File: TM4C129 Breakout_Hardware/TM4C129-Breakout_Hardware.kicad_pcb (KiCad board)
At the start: 2 copper layers, 63.5 x 47 mm, 51 parts, among them J1 RJ45, J2 Conn_02x08, J3 Conn_02x08, J4 Conn_02x08, J5 Conn_02x02, J6 Conn_02x02, U1 HX1198FNL, U2 TM4C129ENCPDT, Y1 NX3225GA, Y2 Crystal 32K SMD

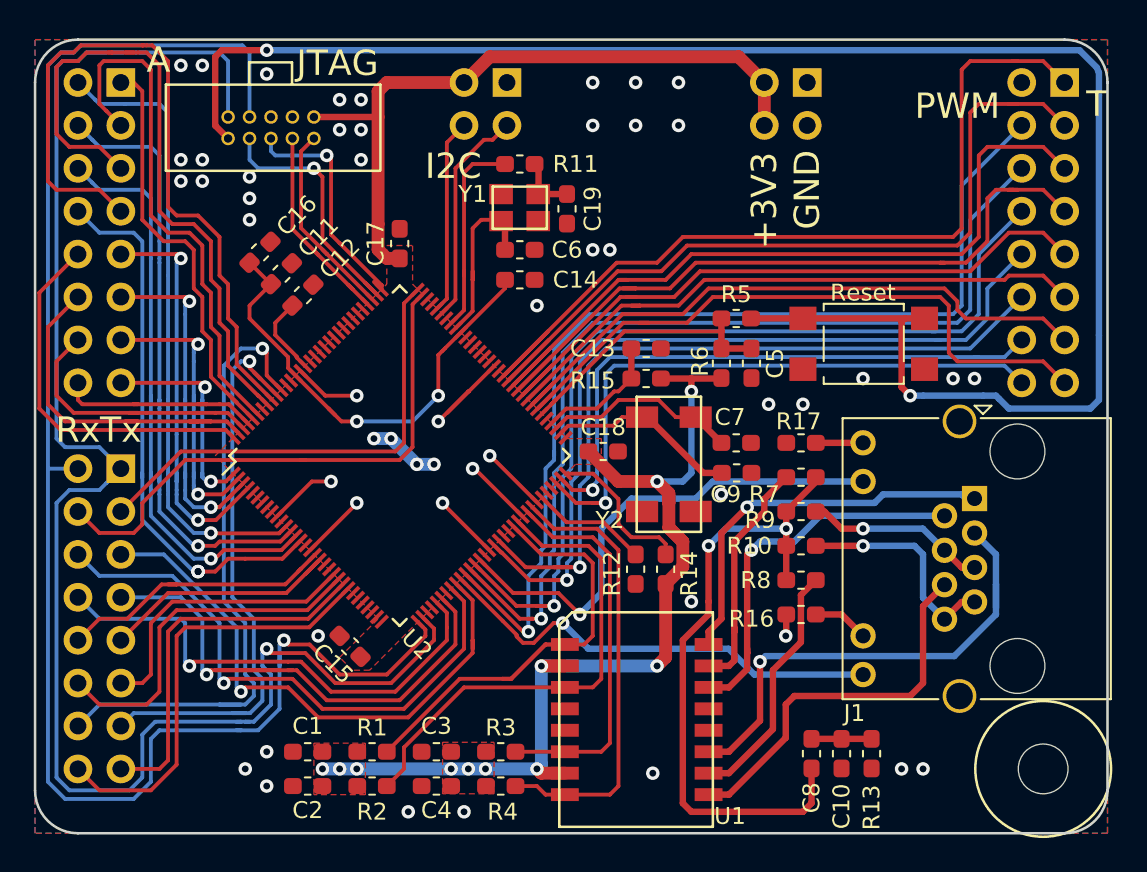
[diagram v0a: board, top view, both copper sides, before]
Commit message: Revert "Revert "Merge branch 'master' of https://github.com/MissouriMRDT/TM4C129-Breakout_Hardware""
This reverts commit 4686fe645caf3e9fbf8c00f0c0ea95986b0ea6b8.
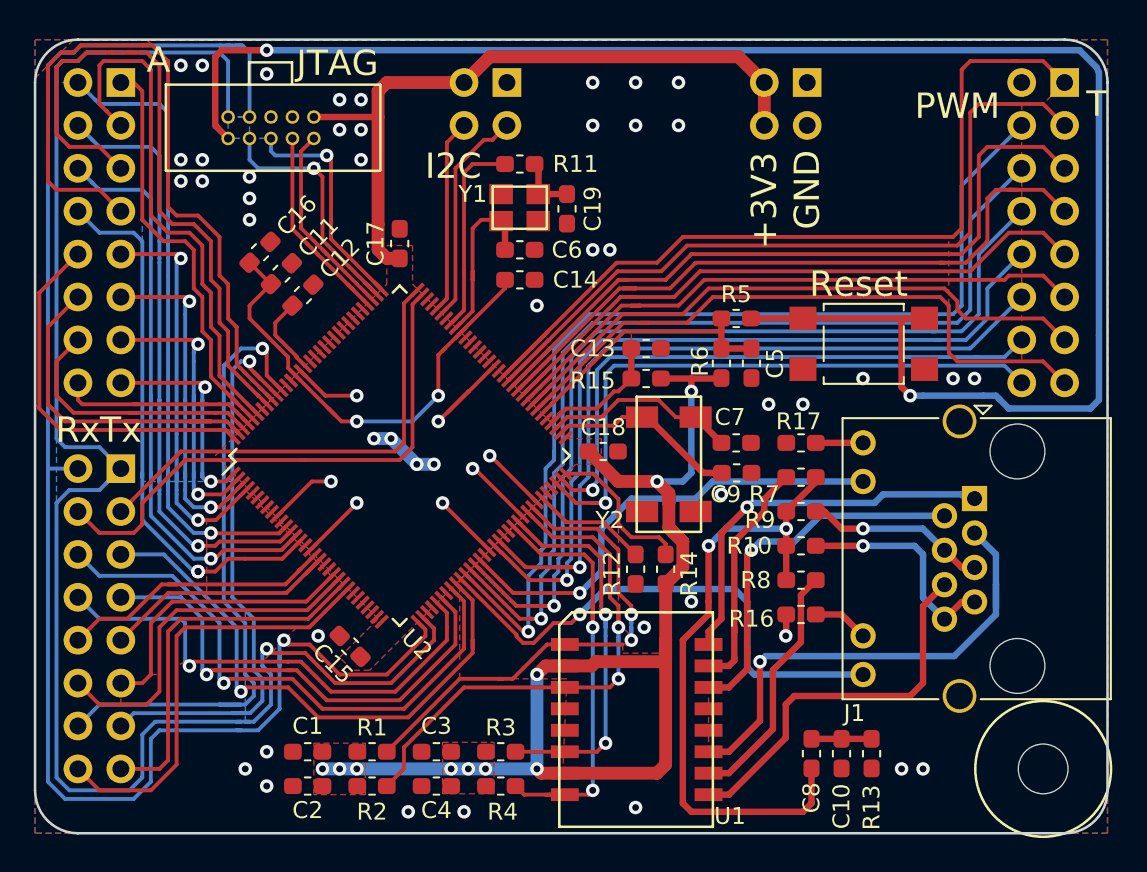
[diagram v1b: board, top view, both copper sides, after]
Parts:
- C14: value .1uF -> 1uF
- SW1: renamed from Reset; value SW_Push -> Reset
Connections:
- R1 pad 2: EN0RXI_N -> EN0TXO_P
- R2 pad 2: EN0RXI_P -> EN0TXO_N
- R3 pad 2: EN0TXO_N -> EN0RXI_P
- R4 pad 2: EN0TXO_P -> EN0RXI_N
- U1 pad 1: EN0RXI_N -> EN0TXO_P
- U1 pad 3: EN0RXI_P -> EN0TXO_N
- U1 pad 6: EN0TXO_N -> EN0RXI_P
- U1 pad 8: EN0TXO_P -> EN0RXI_N
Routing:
- net +3V3: track 109.4 -> 121.3 mm, vias 15 -> 14
- net EN0TXO_N: track 22.9 -> 31.9 mm, vias 0 -> 2
- net EN0RXI_P: track 29.0 -> 23.1 mm, vias 0 -> 2
- net Ethernet_Link: track 27.2 -> 31.2 mm
- net EN0TXO_P: track 26.6 -> 29.8 mm, vias 0 -> 2
- net Ethernet_Activity: track 29.5 -> 27.7 mm
- net EN0RXI_N: track 25.0 -> 26.0 mm, vias 0 -> 2
- net GND: vias 48 -> 49
- added copper zone on B.Cu, net (none)
- added copper zone on F.Cu, net (none)
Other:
- board text added: "Reset"

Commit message: Revert "Merge branch 'master' of https://github.com/MissouriMRDT/TM4C129-Breakout_Hardware"
This reverts commit e6cd920ed13198a4f7d11fd6171e0ba52050bff9, reversing
changes made to e15dd7d36717f2d892901729c8f3941fb424f385.
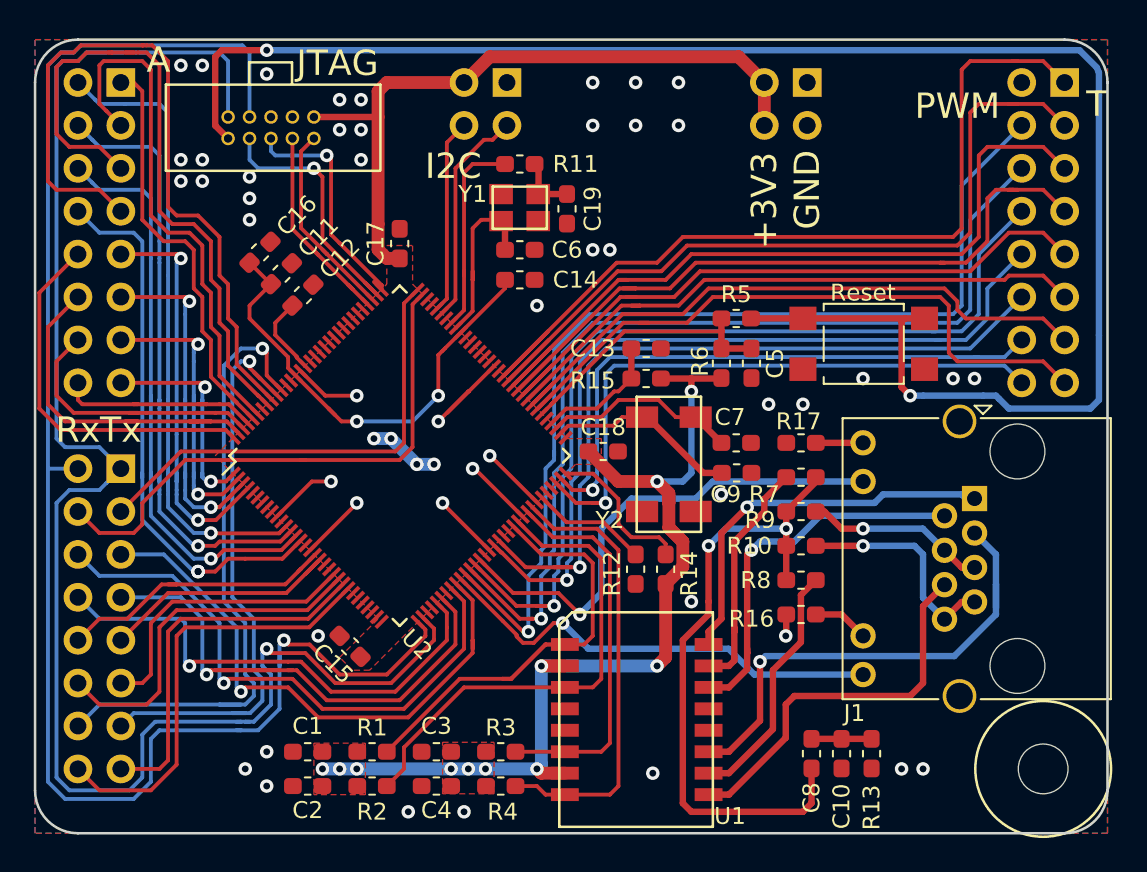
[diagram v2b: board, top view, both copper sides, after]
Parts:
- C14: value 1uF -> .1uF
- Reset: renamed from SW1; value Reset -> SW_Push
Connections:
- R1 pad 2: EN0TXO_P -> EN0RXI_N
- R2 pad 2: EN0TXO_N -> EN0RXI_P
- R3 pad 2: EN0RXI_P -> EN0TXO_N
- R4 pad 2: EN0RXI_N -> EN0TXO_P
- U1 pad 1: EN0TXO_P -> EN0RXI_N
- U1 pad 3: EN0TXO_N -> EN0RXI_P
- U1 pad 6: EN0RXI_P -> EN0TXO_N
- U1 pad 8: EN0RXI_N -> EN0TXO_P
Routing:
- net +3V3: track 121.3 -> 109.4 mm, vias 14 -> 15
- net EN0TXO_N: track 31.9 -> 22.9 mm, vias 2 -> 0
- net EN0RXI_P: track 23.1 -> 29.0 mm, vias 2 -> 0
- net Ethernet_Link: track 31.2 -> 27.2 mm
- net EN0TXO_P: track 29.8 -> 26.6 mm, vias 2 -> 0
- net Ethernet_Activity: track 27.7 -> 29.5 mm
- net EN0RXI_N: track 26.0 -> 25.0 mm, vias 2 -> 0
- net GND: vias 49 -> 48
- removed copper zone on B.Cu, net (none)
- removed copper zone on F.Cu, net (none)
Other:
- board text removed: "Reset"
